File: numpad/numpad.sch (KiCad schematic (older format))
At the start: 35 parts

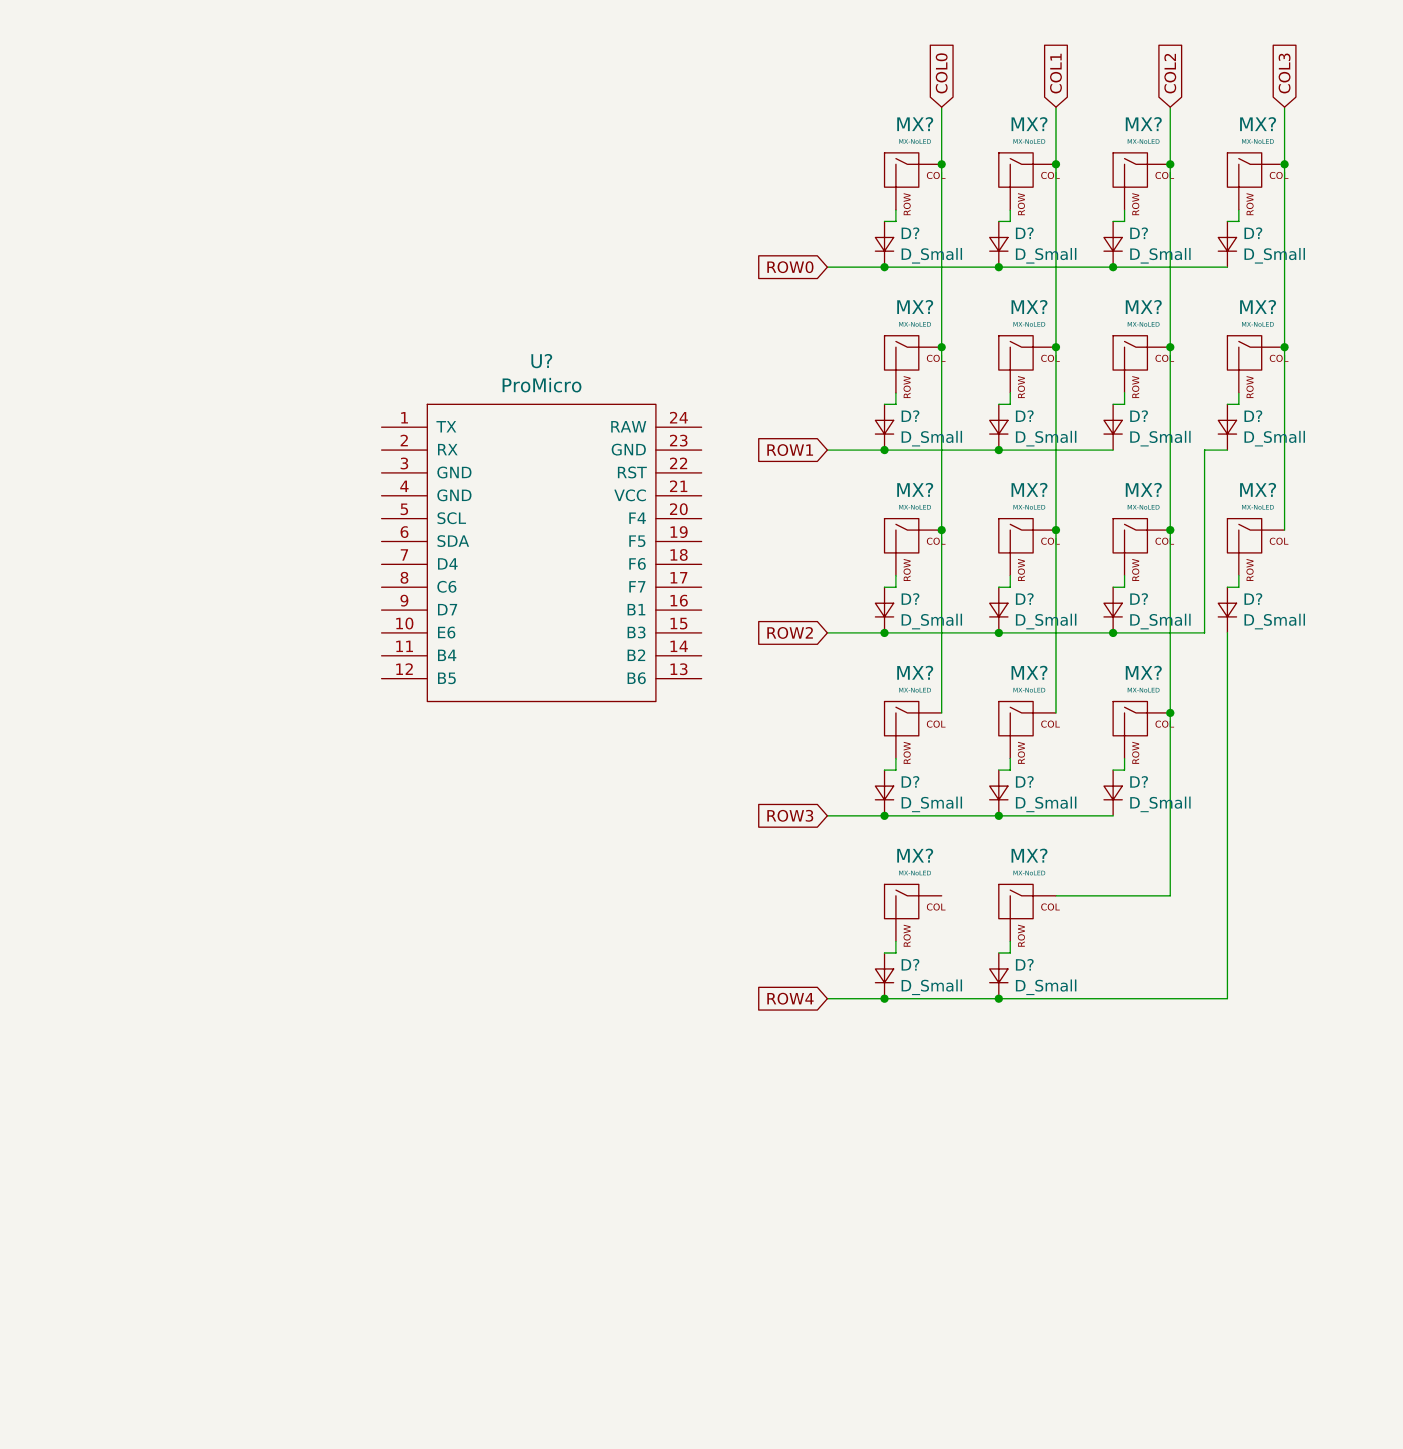
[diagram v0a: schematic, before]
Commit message: Beginning progress, getting there with the schematic
Also got better submodules or whatever they are
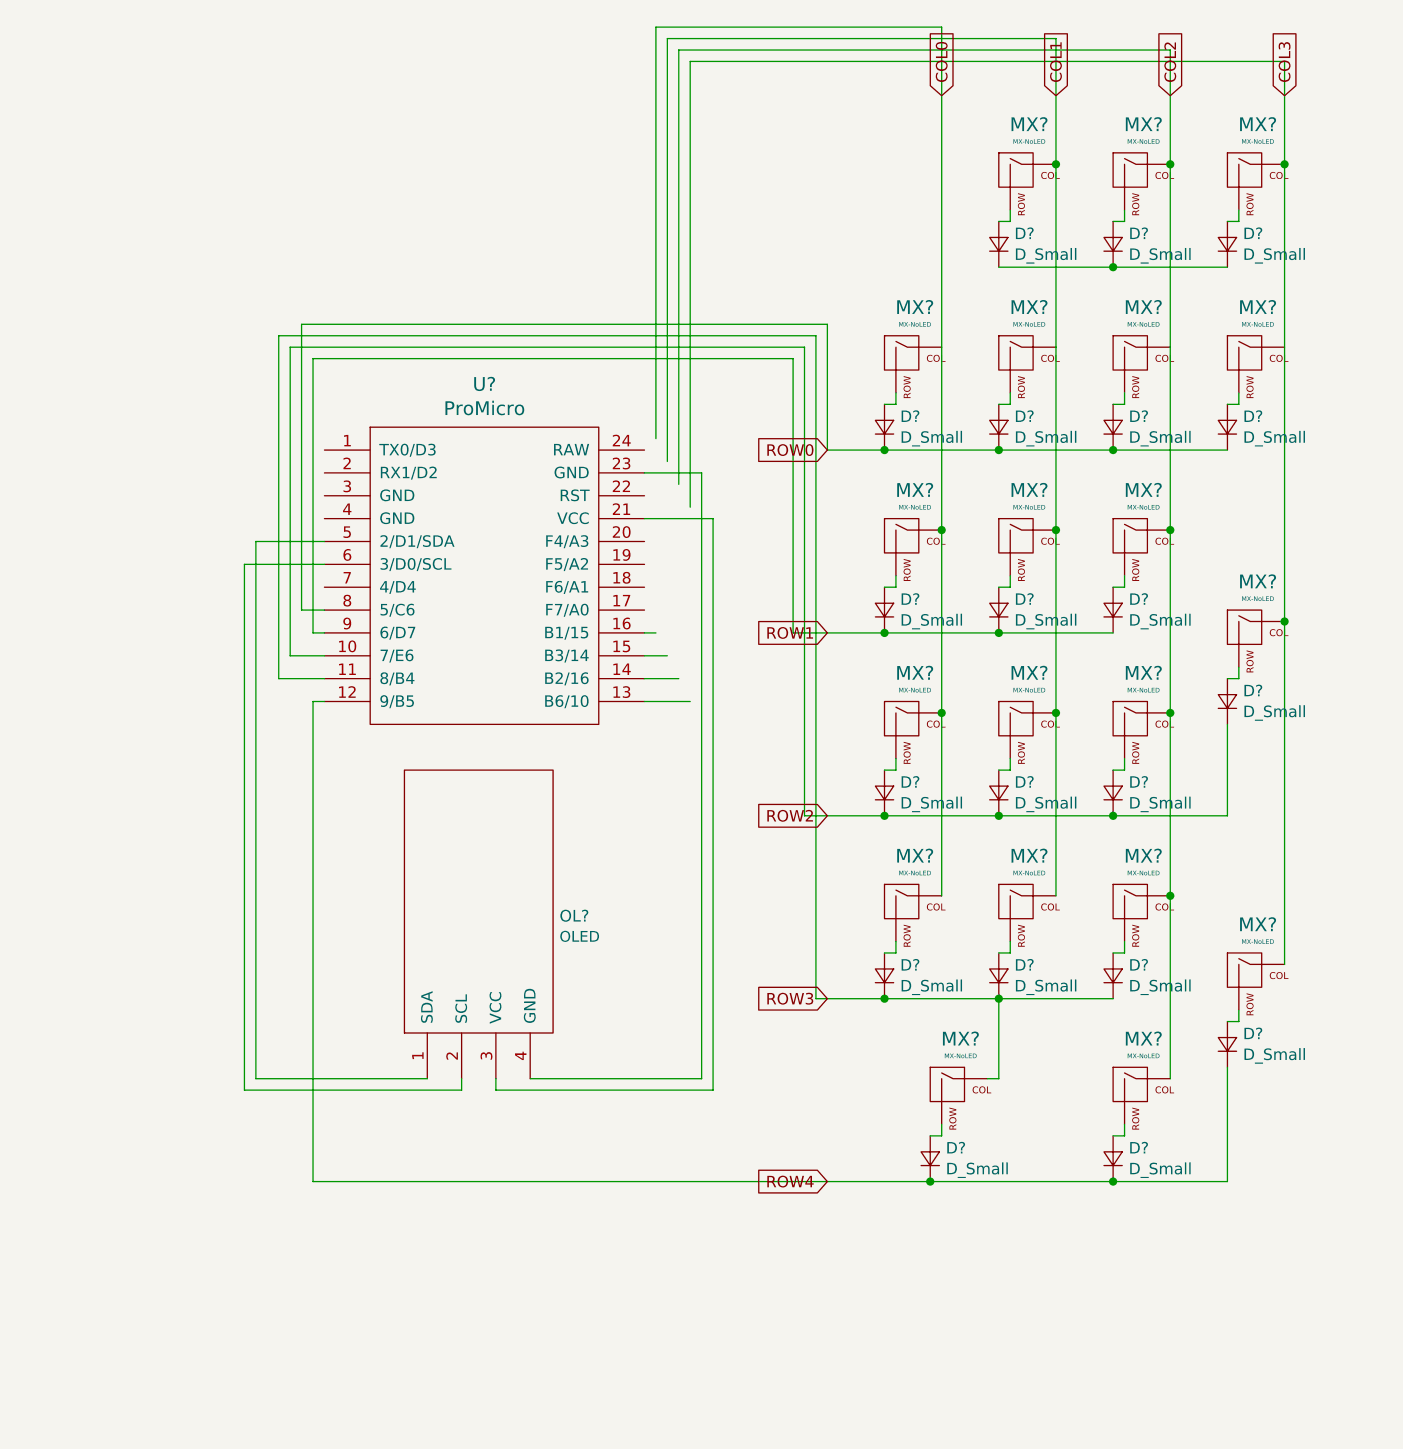
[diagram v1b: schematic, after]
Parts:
- removed U?: ProMicro, symbol promicro:ProMicro
- added D? (x3): D_Small, symbol Device:D_Small
- added MX? (x3): MX-NoLED, symbol MX_Alps_Hybrid:MX-NoLED
- added OL?: OLED, symbol kbd:OLED
- added U?: ProMicro, symbol kbd:ProMicro
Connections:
- wire segments 71 -> 125
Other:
- moved on the sheet: D?, MX?

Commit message: Learned what a fucking global label is
Why the hell did i not know what that does i thought it just looked cool
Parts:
- removed MX? (x20): MX-NoLED, symbol MX_Alps_Hybrid:MX-NoLED
- added D?: D_Small, symbol Device:D_Small
- added MX? (x13), MX_*, MX_-, MX_/, MX_=, MX_BckSpc, MX_Esc, MX_NLck, MX_Tab: MX-LED, symbol MX_Alps_Hybrid:MX-LED
- added R? (x23): R_Small, symbol Device:R_Small
- added SW?: Rotary_Encoder_Switch, symbol Device:Rotary_Encoder_Switch
- added SW?: SW_PUSH, symbol kbd:SW_PUSH
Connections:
- net labels added: ENCA, ENCB, GND, LED, ROW5, RST, SCL, SDA, VCC
- wire segments 125 -> 169
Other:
- moved on the sheet: D?, OL?, U?
